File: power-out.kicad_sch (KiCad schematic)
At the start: 1 part, among them U2 TPS61022

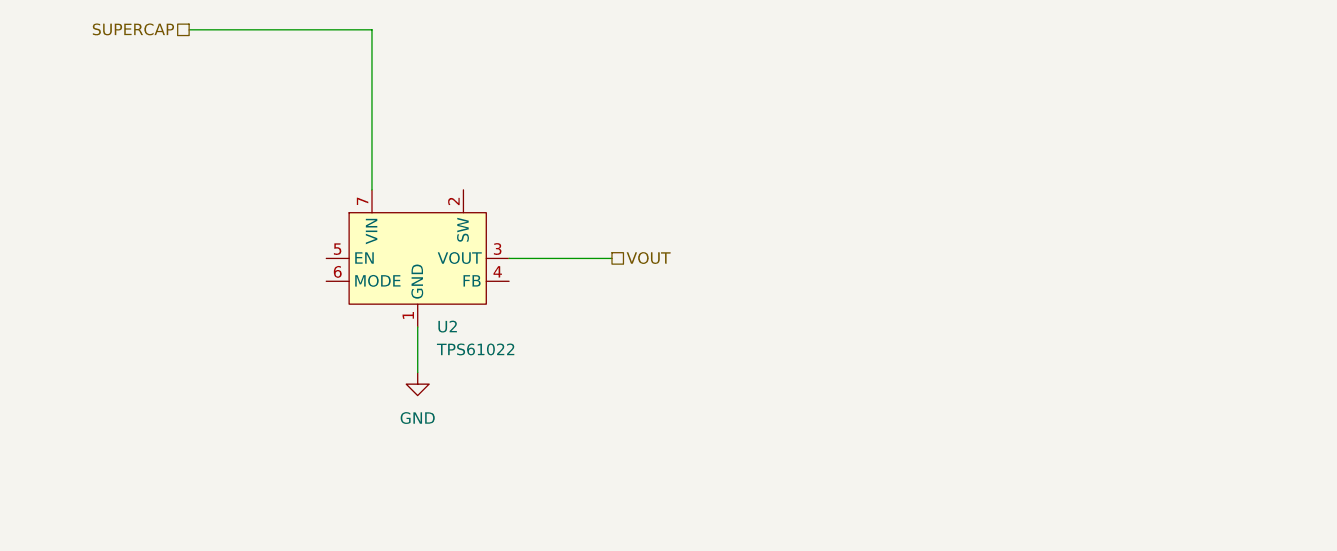
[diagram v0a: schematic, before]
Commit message: Configure power output
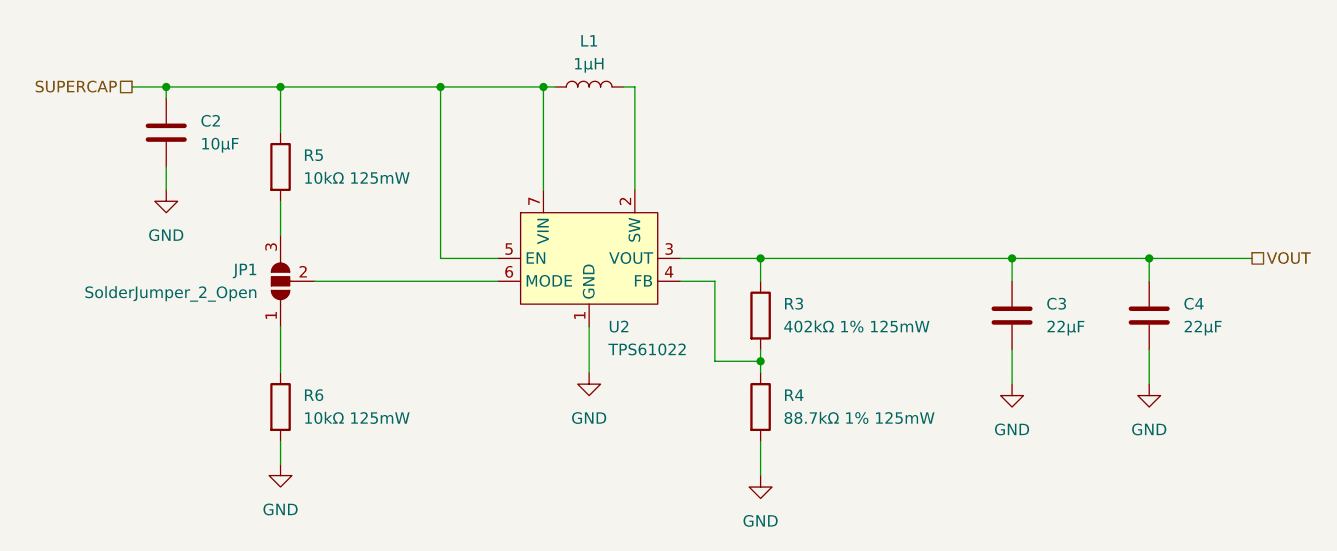
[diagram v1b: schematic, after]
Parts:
- added C2: 10µF, symbol Device:C
- added C3, C4: 22µF, symbol Device:C
- added JP1: SolderJumper_2_Open, Jumper:SolderJumper-3_P1.3mm_Open_RoundedPad1.0x1.5mm_NumberLabels, symbol Jumper:SolderJumper_3_Open
- added L1: 1µH, symbol Device:L
- added R3: 402kΩ 1% 125mW, Resistor_SMD:R_0805_2012Metric_Pad1.20x1.40mm_HandSolder, symbol Device:R
- added R4: 88.7kΩ 1% 125mW, Resistor_SMD:R_0805_2012Metric_Pad1.20x1.40mm_HandSolder, symbol Device:R
- added R5, R6: 10kΩ 125mW, Resistor_SMD:R_0805_2012Metric_Pad1.20x1.40mm_HandSolder, symbol Device:R
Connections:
- net GND: now also C2.2, C3.2, C4.2, R4.2, R6.2
- net SUPERCAP: now also U2.5 (EN), C2.1, L1.1, R5.1
- net VOUT: now also C3.1, C4.1, R3.1
- net at U2.2 (SW): now also L1.2
- net at U2.4 (FB): now also R3.2, R4.1
- net at U2.6 (MODE): now also JP1.2 (C)
- new net: JP1.3 (B), R5.2
- new net: JP1.1 (A), R6.1
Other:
- moved on the sheet: U2
